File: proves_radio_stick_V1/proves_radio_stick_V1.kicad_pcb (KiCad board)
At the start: 4 copper layers, 88.2 x 94.5 mm, 53 parts, among them J1 SWD Port, J12 USB_C_Receptacle_USB2.0_16P, J22 SWD Port, SW1 KMR2, SW2 KMR2, U11 W25Q128JVS, U18 RP2350_60QFN, U2 TPS62085RLTT, U3 E32-400M20S_C2965514, Y1 ABM8-272-T3

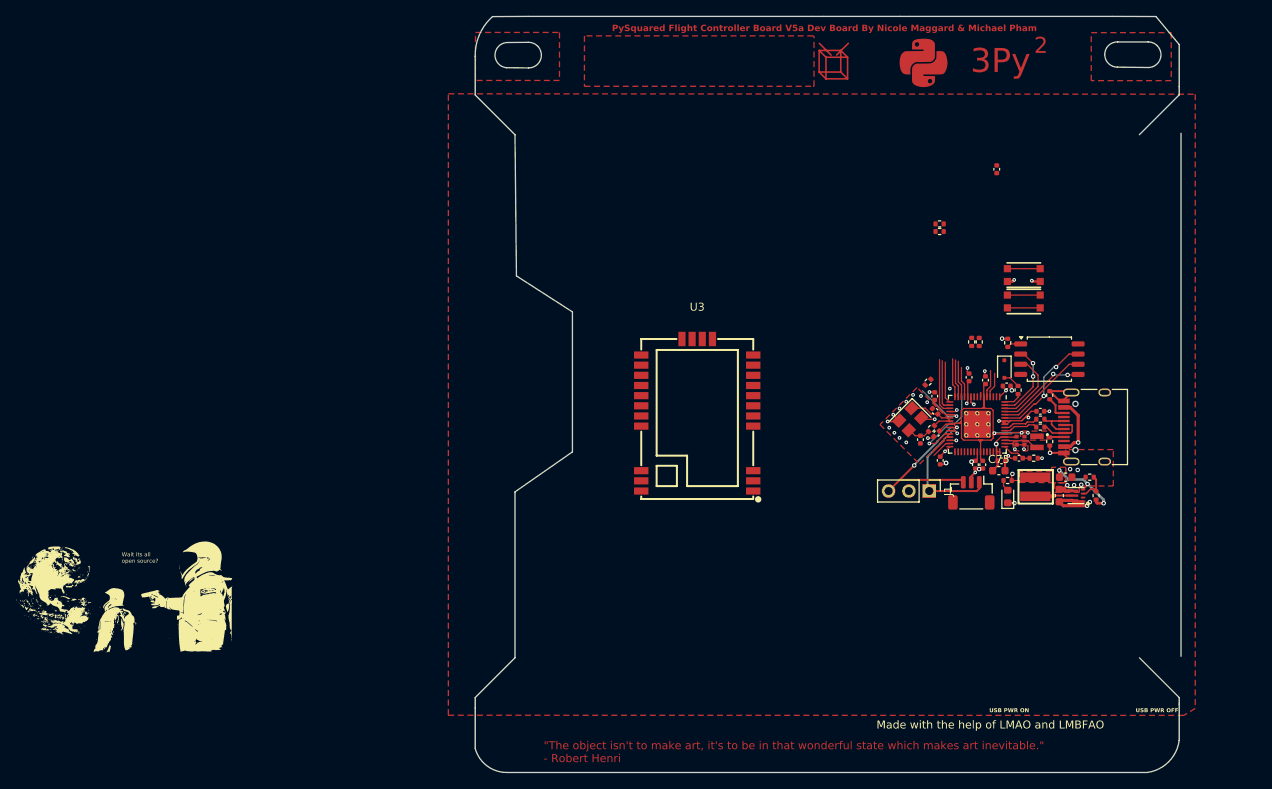
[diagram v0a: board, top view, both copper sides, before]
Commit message: Initial Layout Complete
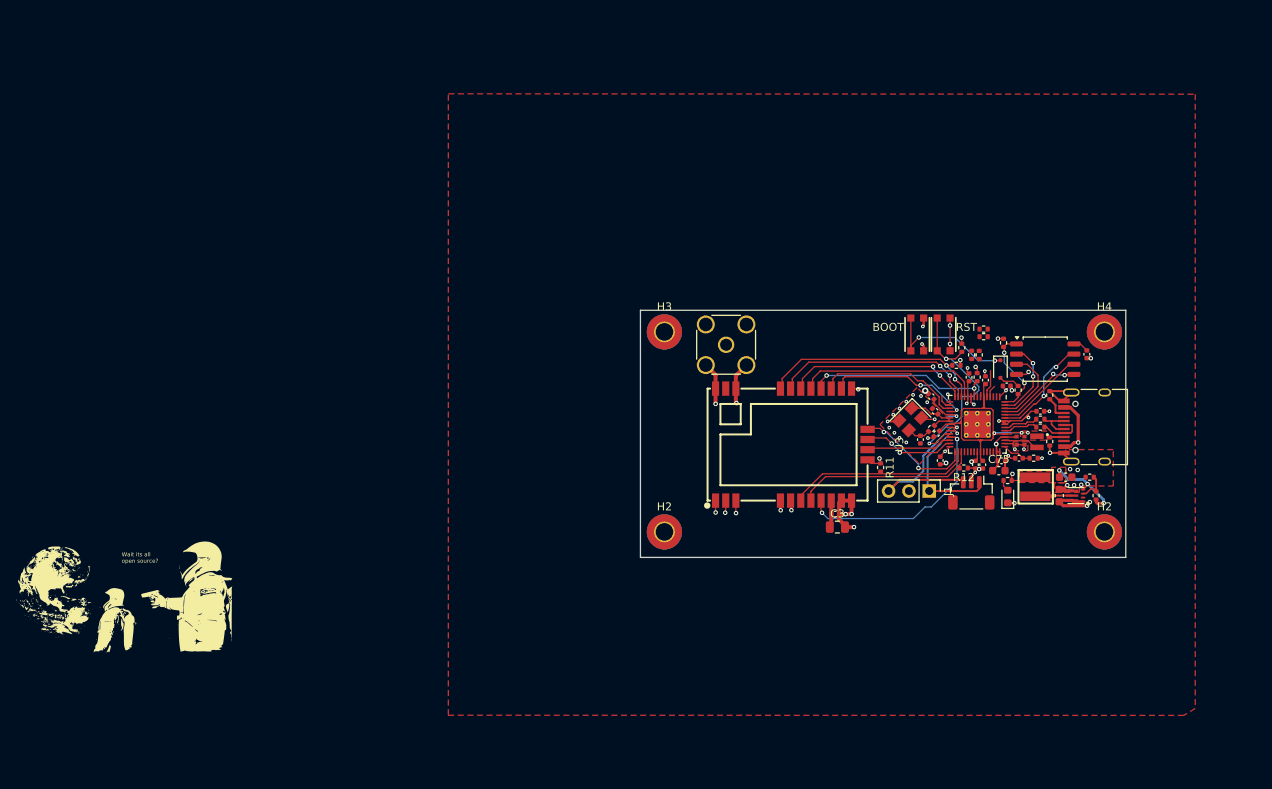
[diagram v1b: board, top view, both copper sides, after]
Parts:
- removed the G*** at (199.4, 54.0) (x2)
- removed the G*** at (171.0, 53.0)
- added C1: 100n, Capacitor_SMD:C_0402_1005Metric, F.Cu at (188.3, 109.8)
- added C3: 47uF, Capacitor_SMD:C_0805_2012Metric, F.Cu at (188.6, 111.4)
- added H2: MountingHole, MountingHole:MountingHole_2.2mm_M2_Pad_TopBottom, F.Cu at (222.0, 112.0)
- added H2: MountingHole, MountingHole:MountingHole_2.2mm_M2_Pad_TopBottom, F.Cu at (167.0, 112.0)
- added H3: MountingHole, MountingHole:MountingHole_2.2mm_M2_Pad_TopBottom, F.Cu at (167.0, 87.0)
- added H4: MountingHole, MountingHole:MountingHole_2.2mm_M2_Pad_TopBottom, F.Cu at (222.0, 87.0)
- added J2: Conn_Coaxial, Connector_Coaxial:SMA_Amphenol_132134_Vertical, F.Cu at (174.7, 88.6)
- added R11: 10k, Resistor_SMD:R_0402_1005Metric, F.Cu at (194.0, 104.0)
- added R12: 10k, Resistor_SMD:R_0402_1005Metric, F.Cu at (204.4, 104.0)
- added R5: 10k, Resistor_SMD:R_0402_1005Metric, F.Cu at (206.1, 92.7)
- added R9: 10k, Resistor_SMD:R_0402_1005Metric, F.Cu at (203.5, 91.2)
- moved C2 25.7 mm to (219.8, 89.8), turned to -90 degrees
- moved SW1 15.2 mm to (198.6, 87.3), turned to 90 degrees
- moved R6 14.3 mm to (206.9, 86.7)
- moved R25 14.3 mm to (206.9, 87.6)
- moved U3 12.4 mm to (182.9, 101.1), turned to -90 degrees
- moved SW2 10.8 mm to (201.9, 87.3), turned to 90 degrees
- moved R1 6.02 mm to (204.2, 89.0), turned to -90 degrees
- moved R39 1.62 mm to (205.4, 89.9)
- moved R41 1.62 mm to (206.3, 89.9)
- moved R2 0.52 mm to (209.4, 88.4)
- moved U11 0.52 mm to (214.6, 90.4)
- moved D4 0.49 mm to (209.0, 91.6)
- moved C71 0.43 mm to (200.4, 95.1), turned to 135 degrees
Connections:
- R2 pad 2: /FLASH_SS -> BOOTSEL
- U11 pad 1: /FLASH_SS -> BOOTSEL
- U18 pad 10: SPI1_CS0 -> unconnected-(U18-GPIO7-Pad10)
- U18 pad 12: SPI0_MISO -> SPI1_MISO
- U18 pad 13: SPI0_CS0 -> SPI1_CS0
- U18 pad 14: SPI0_SCK -> SPI1_SCK
- U18 pad 15: SPI0_MOSI -> SPI1_MOSI
- U18 pad 16: RF1_IO4 -> unconnected-(U18-GPIO12-Pad16)
- U18 pad 17: RF1_IO0 -> unconnected-(U18-GPIO13-Pad17)
- U18 pad 18: RF2_IO3 -> RF1_IO0
- U18 pad 19: SPI1_CS1 -> RF1_IO1
- U18 pad 27: SPI1_MISO -> RF1_IO2
- U18 pad 28: RF2_RST -> RF1_IO3
- U18 pad 29: SPI1_SCK -> RF1_IO4
- U18 pad 31: SPI1_MOSI -> RF1_IO5
- U18 pad 32: ~{GPIO_EXPANDER_RESET} -> RF1_RX_EN
- U18 pad 33: RF2_RX_EN -> RF1_TX_EN
- U18 pad 34: RF2_TX_EN -> unconnected-(U18-GPIO22-Pad34)
- U18 pad 35: RF2_IO0 -> unconnected-(U18-GPIO23-Pad35)
- U18 pad 36: WDT_WDI -> unconnected-(U18-GPIO24-Pad36)
- U18 pad 37: WDT_ENABLE -> unconnected-(U18-GPIO25-Pad37)
- U18 pad 40: ~{MUX_RESET} -> unconnected-(U18-GPIO26_ADC0-Pad40)
- U18 pad 41: RTC_INT -> unconnected-(U18-GPIO27_ADC1-Pad41)
- U18 pad 42: ~{FIRE_DEPLOY1_A} -> unconnected-(U18-GPIO28_ADC2-Pad42)
- U18 pad 43: ~{FIRE_DEPLOY1_B} -> unconnected-(U18-GPIO29_ADC3-Pad43)
- U3 pad 1: unconnected-(U3-GND-Pad1) -> GND
- U3 pad 10: unconnected-(U3-GND-Pad10) -> GND
- U3 pad 11: unconnected-(U3-GND-Pad11) -> GND
- U3 pad 12: unconnected-(U3-GND-Pad12) -> GND
- U3 pad 13: unconnected-(U3-DIO3-Pad13) -> RF1_IO3
- U3 pad 14: unconnected-(U3-DIO4-Pad14) -> RF1_IO4
- U3 pad 15: unconnected-(U3-DIO5-Pad15) -> RF1_IO5
- U3 pad 16: unconnected-(U3-GND-Pad16) -> GND
- U3 pad 17: unconnected-(U3-DIO1-Pad17) -> RF1_IO1
- U3 pad 18: unconnected-(U3-DIO0-Pad18) -> RF1_IO0
- U3 pad 19: unconnected-(U3-RST-Pad19) -> RF1_RST
- U3 pad 2: unconnected-(U3-GND-Pad2) -> GND
- U3 pad 20: unconnected-(U3-MISO-Pad20) -> SPI1_MISO
- U3 pad 21: unconnected-(U3-MOSI-Pad21) -> SPI1_MOSI
- U3 pad 22: unconnected-(U3-SCK-Pad22) -> SPI1_SCK
- U3 pad 23: unconnected-(U3-NSS-Pad23) -> SPI1_CS0
- U3 pad 24: unconnected-(U3-GND-Pad24) -> GND
- U3 pad 25: unconnected-(U3-ANT-Pad25) -> Net-(J2-In)
- U3 pad 26: unconnected-(U3-GND-Pad26) -> GND
- U3 pad 3: unconnected-(U3-GND-Pad3) -> GND
- U3 pad 4: unconnected-(U3-GND-Pad4) -> GND
- U3 pad 5: unconnected-(U3-GND-Pad5) -> GND
- U3 pad 6: unconnected-(U3-RXEN-Pad6) -> RF1_RX_EN
- U3 pad 7: unconnected-(U3-TXEN-Pad7) -> RF1_TX_EN
- U3 pad 8: unconnected-(U3-DIO2-Pad8) -> RF1_IO2
- U3 pad 9: unconnected-(U3-VCC-Pad9) -> +3V3
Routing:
- net GND: track 53.0 -> 85.3 mm, vias 33 -> 50
- net RF1_IO2: track 0.00 -> 27.3 mm, vias 0 -> 2
- net SPI1_CS0: track 1.56 -> 28.4 mm, vias 1 -> 2
- net RF1_RX_EN: track 0.00 -> 23.3 mm
- net RF1_RST: track 0.00 -> 23.2 mm, vias 0 -> 2
- net SPI1_SCK: track 2.56 -> 25.4 mm, vias 0 -> 2
- net RF1_TX_EN: track 0.00 -> 22.8 mm
- net SPI1_MOSI: track 0.10 -> 22.9 mm, vias 0 -> 2
- net SPI1_MISO: track 3.14 -> 22.9 mm
- net RF1_IO1: track 0.00 -> 18.1 mm, vias 0 -> 2
- net RF1_IO5: track 0.00 -> 14.8 mm, vias 0 -> 2
- net /USBBOOT: track 4.10 -> 17.6 mm, vias 0 -> 2
- net FC_RESET: track 15.2 -> 27.5 mm, vias 1 -> 2
- net RF1_IO0: track 6.36 -> 18.2 mm
- net RF1_IO3: track 0.00 -> 10.5 mm
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- removed copper zone on F.Cu, net (none)
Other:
- board size 88.2 x 94.5 mm -> 60.7 x 30.9 mm
- board text added: "BOOT"
- board text added: "RST"
- board text removed: "2"
- board text removed: "3Py"
- board text removed: "JLCJLCJLCJLC"
- board text removed: "Made with the help of LMAO and LMBFAO"
- board text removed: "PySquared Flight Controller Board V5a Dev Board By Nicole Maggard & Michael Pham"
- board text removed: "USB PWR OFF"
- board text removed: "USB PWR ON"
- board text removed: "{dblquote}The object isn't to make art, it's to be in that wonderful state which makes art inevitable.{dblquote} - Robert Henri"
